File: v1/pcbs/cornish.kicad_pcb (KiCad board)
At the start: 2 copper layers, 155.9 x 133.8 mm, 90 parts

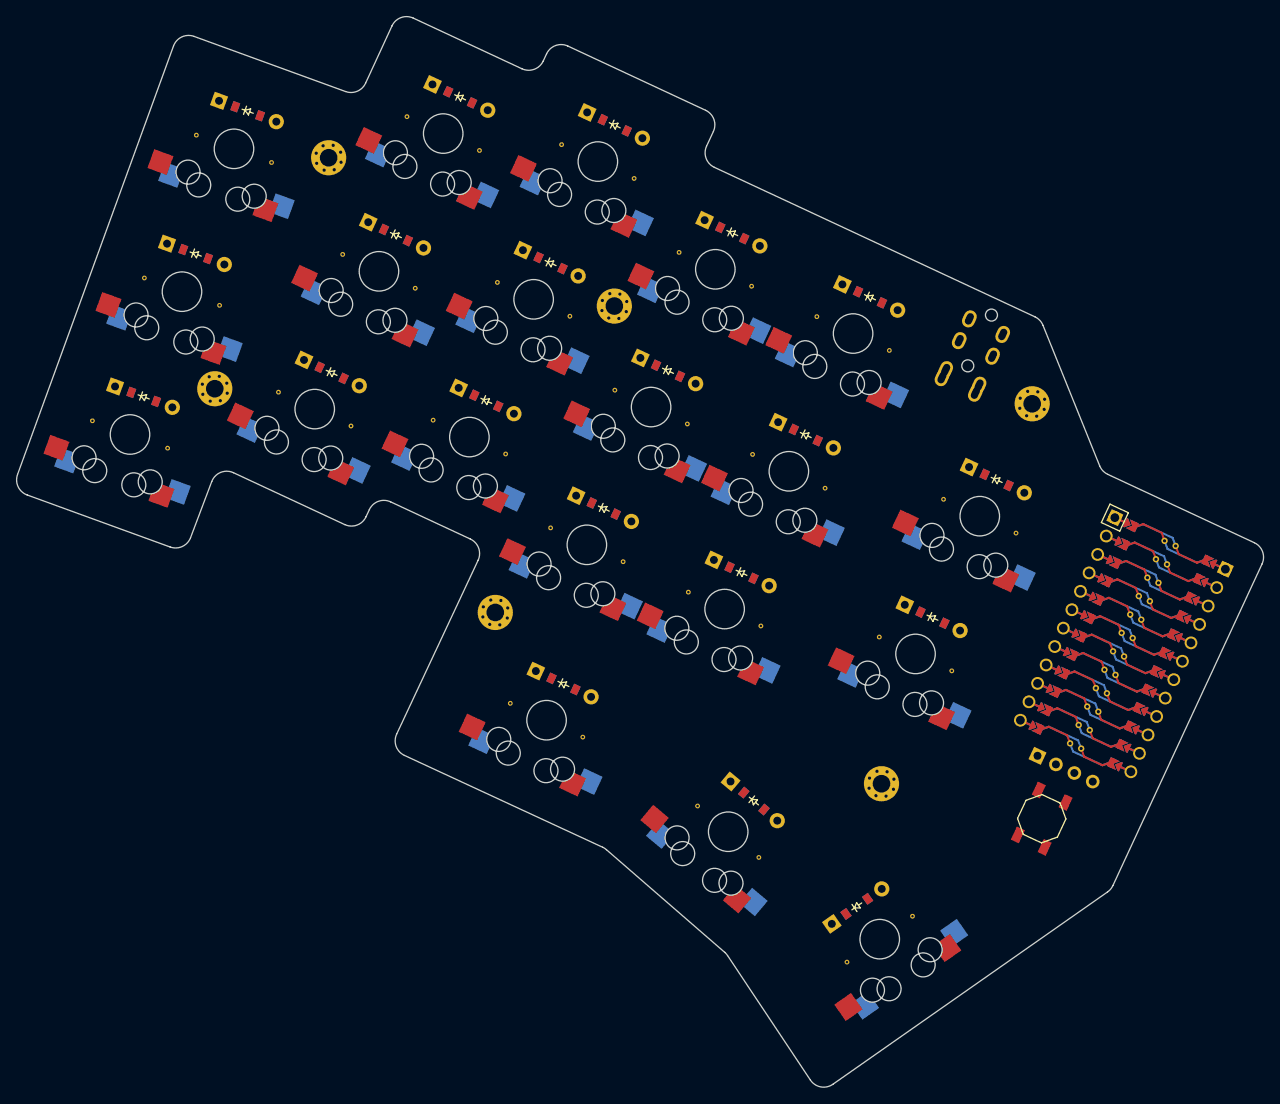
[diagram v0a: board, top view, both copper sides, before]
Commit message: v1.1 and case
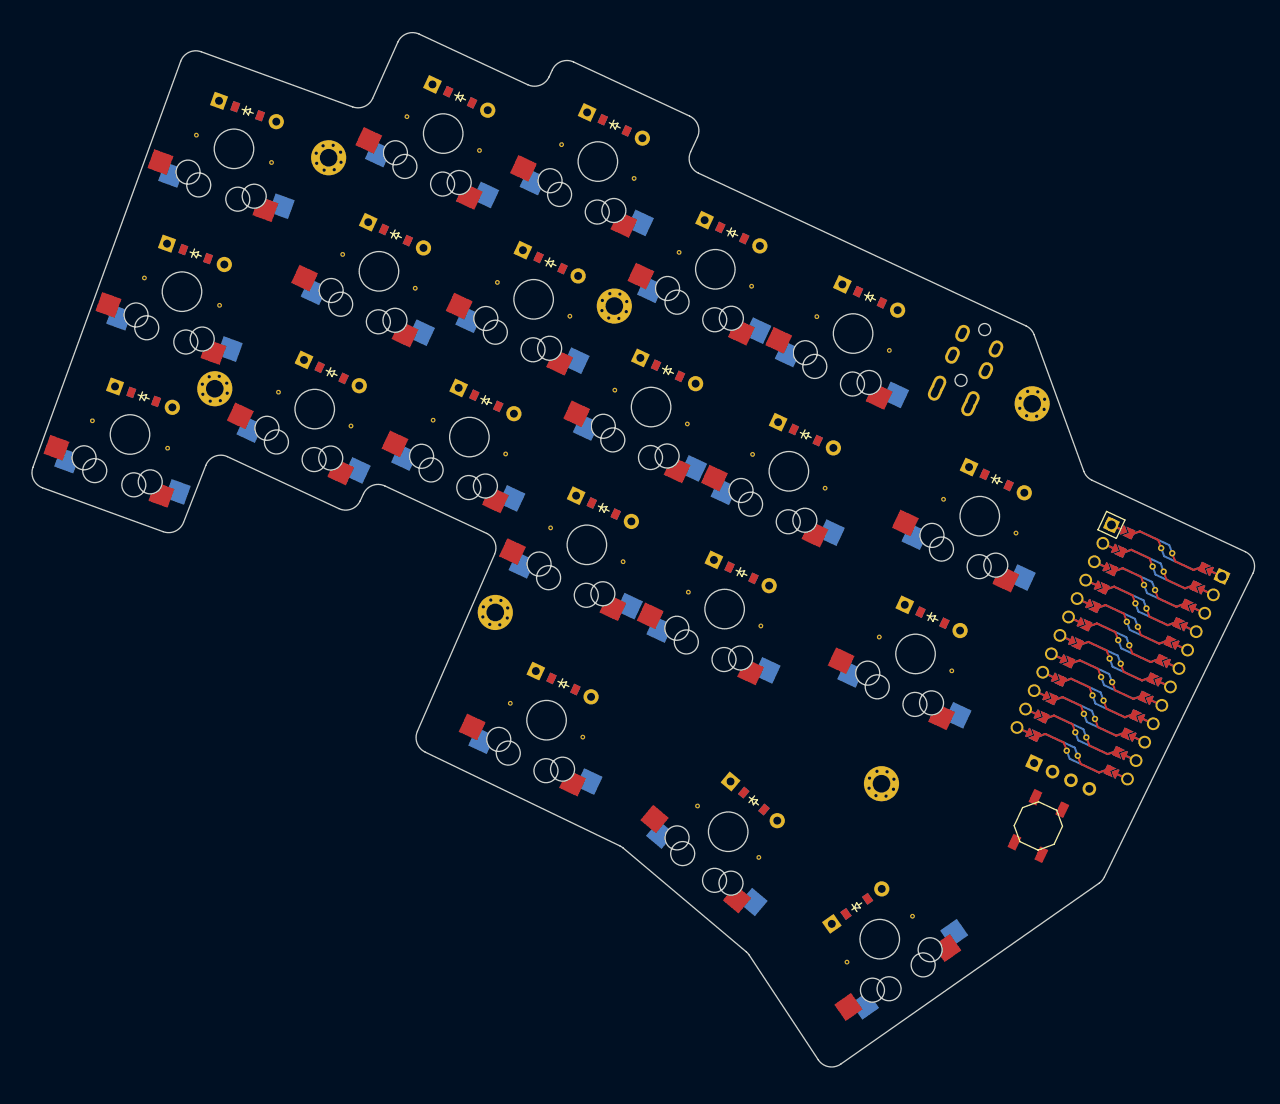
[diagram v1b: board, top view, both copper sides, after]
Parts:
- moved TRRS1 2.00 mm to (254.8, 113.7)
- moved B1 1.00 mm to (258.7, 176.3)
- moved _41 1.00 mm to (268.9, 154.5)
- moved OLED1 1.00 mm to (267.8, 171.1)
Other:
- board size 155.9 x 133.8 mm -> 152.8 x 129.3 mm
